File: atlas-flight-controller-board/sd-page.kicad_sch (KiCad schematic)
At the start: 1 part, among them J1 Conn_01x07_Socket

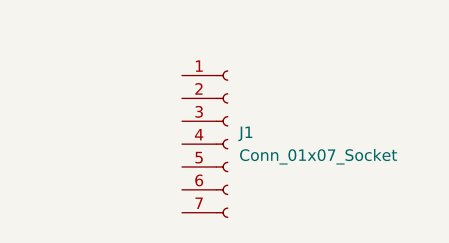
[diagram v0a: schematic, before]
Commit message: finishing up schematic for v1.
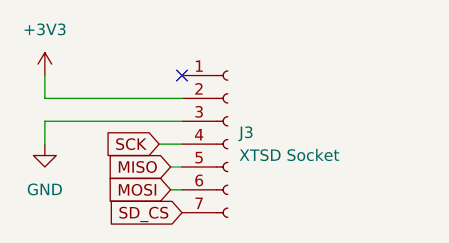
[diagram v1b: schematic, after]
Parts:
- J3: renamed from J1; value Conn_01x07_Socket -> XTSD Socket
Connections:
- net +3V3: now reaches J3.2 (Pin_2)
- net GND: now reaches J3.3 (Pin_3)
- net SCK: now reaches J3.4 (Pin_4)
- net MISO: now reaches J3.5 (Pin_5)
- net MOSI: now reaches J3.6 (Pin_6)
- net SD_CS: now reaches J3.7 (Pin_7)
- no-connect marks 0 -> 1
